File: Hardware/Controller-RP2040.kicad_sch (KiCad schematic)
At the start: 43 parts, among them J1 Conn_01x07_Male, J2 Conn_01x04_Male, J3 Conn_01x02_Male, J4 Conn_01x02_Male, J5 Conn_01x02_Male, J6 Conn_01x02_Male, J7 Conn_01x08_Male, J8 QWIIC_Vertical, J9 QWIIC_Stackable, Q1 DMG1012T, U1 RP2040, U2 W25Q32JVXGIQ, Y1 12MHz

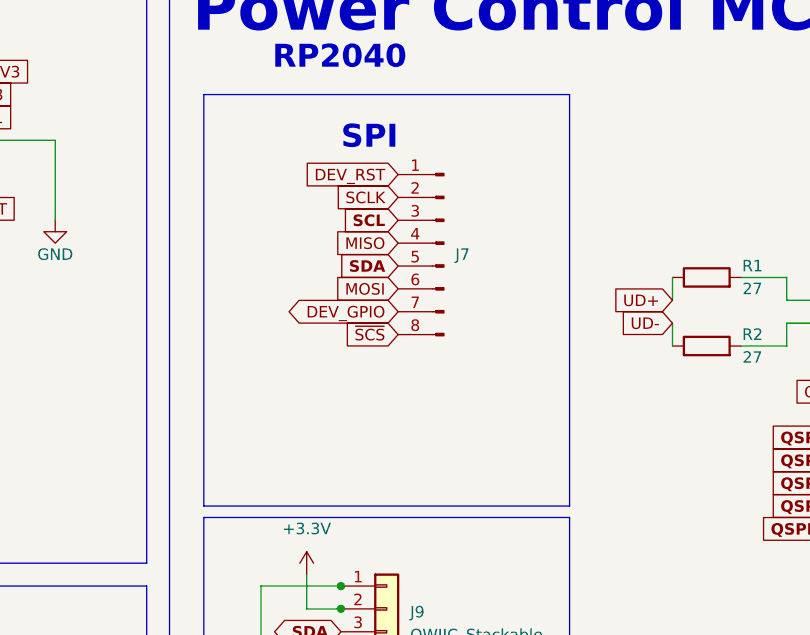
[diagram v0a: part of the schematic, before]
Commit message: Bit more of the RP2040...
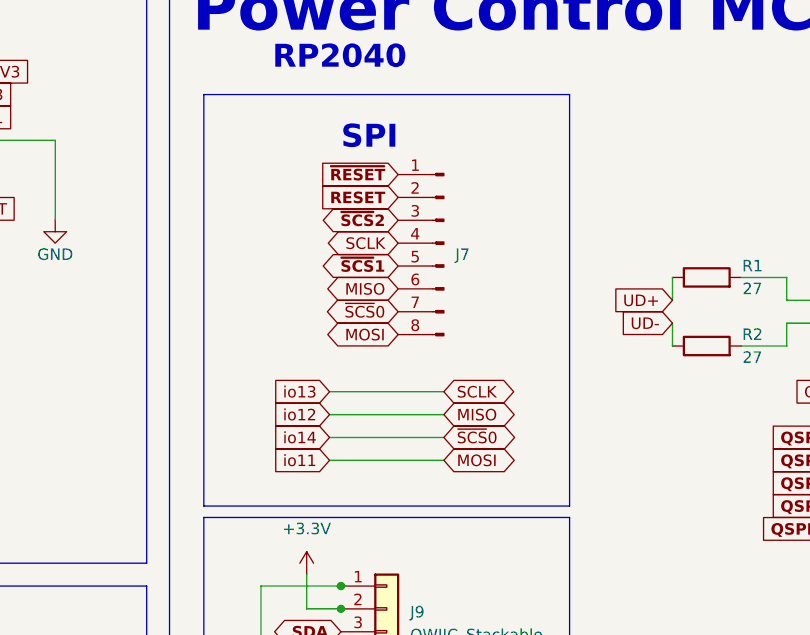
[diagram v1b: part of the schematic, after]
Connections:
- net DEV_GPIO is gone; now on net io14: J7.7 (Pin_7)
- net io11 is gone; now on net MOSI: U1.14 (GPIO11)
- net io12 is gone; now on net MISO: U1.15 (GPIO12)
- net io13 is gone; now on net SCLK: U1.16 (GPIO13)
- net ~{SCS} is gone; now on net MOSI: J7.8 (Pin_8)
- net MISO: now also J7.6 (Pin_6); no longer J7.4 (Pin_4)
- net MOSI: no longer J7.6 (Pin_6)
- net SCL: no longer J7.3 (Pin_3)
- net SCLK: now also J7.4 (Pin_4); no longer J7.2 (Pin_2)
- net SDA: no longer J7.5 (Pin_5)
- net DEV_RST renamed ~{RESET}
- new net RESET: J7.2 (Pin_2)
- new net ~{SCS}1: J7.5 (Pin_5)
- new net ~{SCS}2: J7.3 (Pin_3)
